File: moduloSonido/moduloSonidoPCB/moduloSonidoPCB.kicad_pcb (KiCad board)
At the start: 2 copper layers, 25.4 x 33.8 mm, 11 parts, among them J1 Conn_01x03, J2 Conn_01x05, U1 ATtiny85V-10P

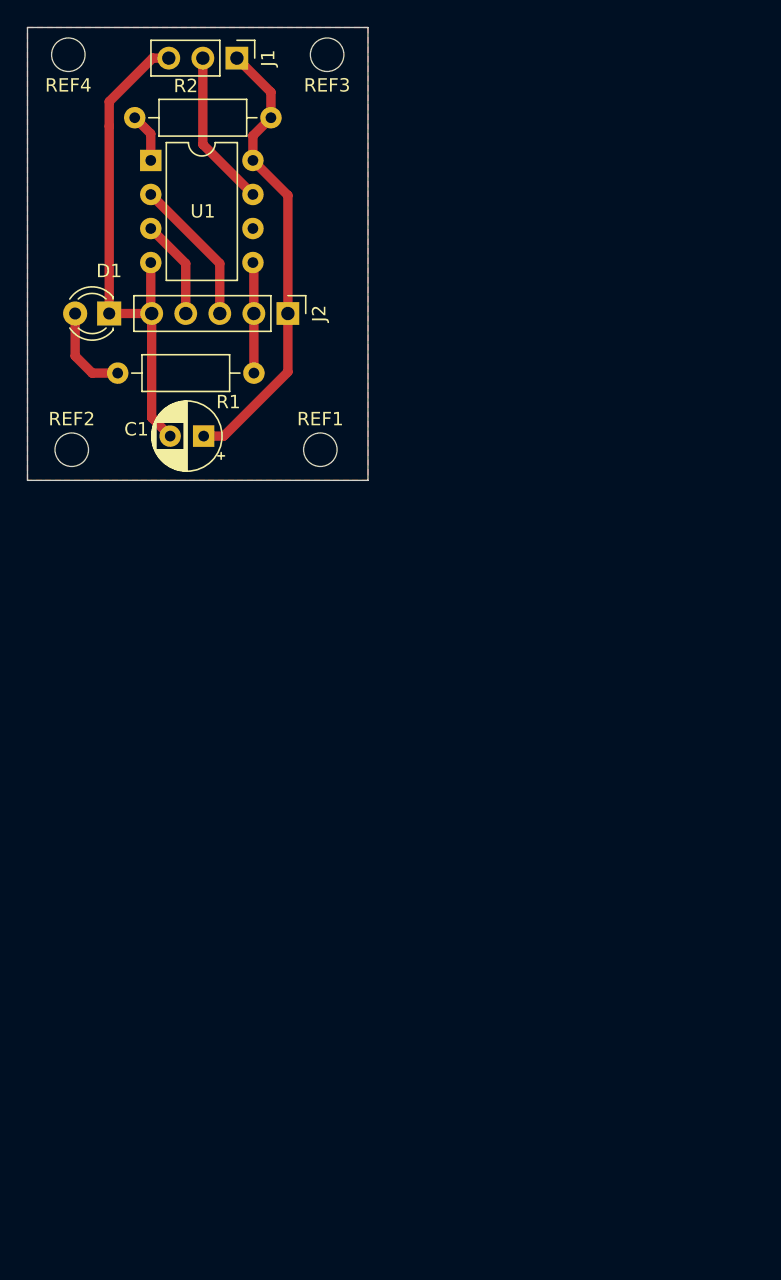
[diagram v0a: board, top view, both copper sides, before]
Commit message: Actualizacion PCB
Algunos cambios en diseño de PCB
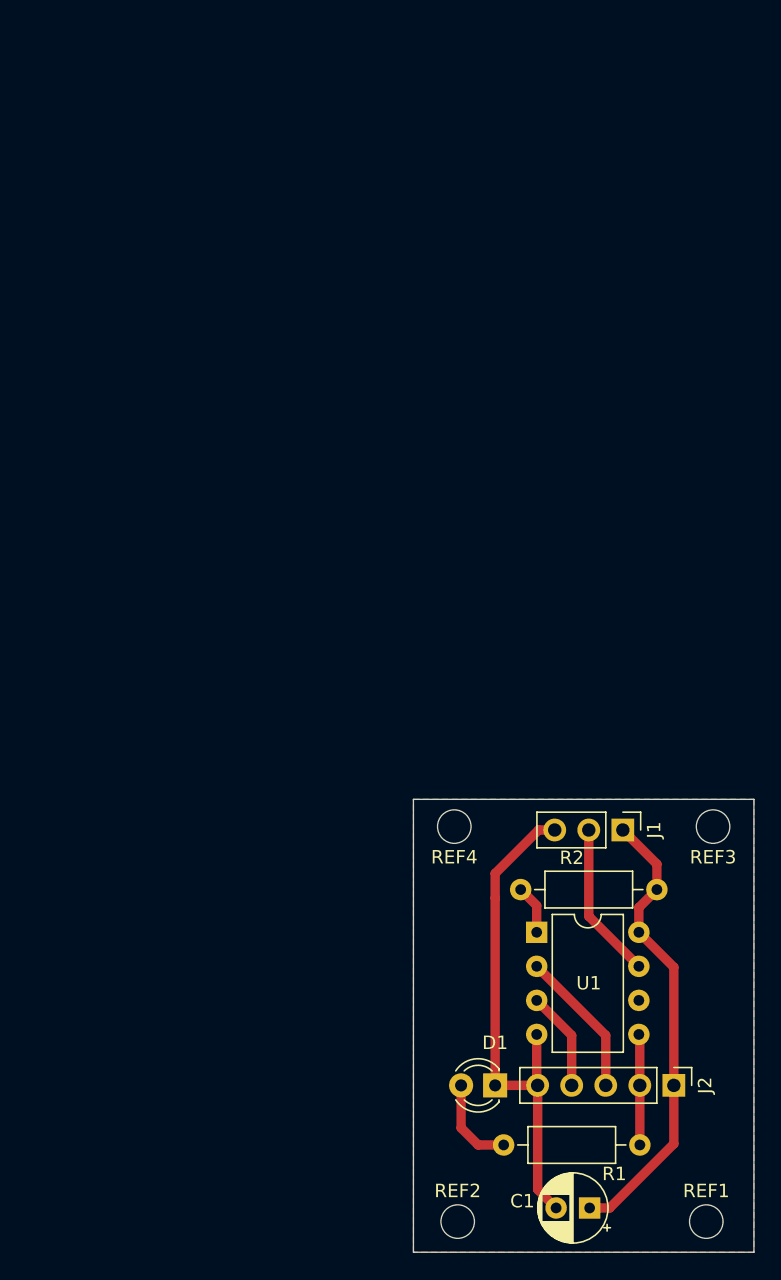
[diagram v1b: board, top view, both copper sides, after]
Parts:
- moved C1 64.4 mm to (129.7, 106.8)
- moved R1 64.4 mm to (133.5, 102.1)
- moved R2 64.4 mm to (124.6, 83.1)
- moved D1 64.4 mm to (122.7, 97.7)
- moved J1 64.4 mm to (132.2, 78.6)
- moved J2 64.4 mm to (136.0, 97.7)
- moved REF1 64.4 mm to (138.4, 107.8)
- moved REF2 64.4 mm to (119.9, 107.8)
- moved REF3 64.4 mm to (138.9, 78.4)
- moved REF4 64.4 mm to (119.6, 78.4)
- moved U1 64.4 mm to (125.8, 86.2)
